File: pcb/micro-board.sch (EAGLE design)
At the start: 116 parts, among them IC1 STM32F401RET6U, IC2 LDS3985M33R, IC3 LDS3985M33R, IC4 HX711, IC5 TLV2462IP, J12 B2B-PH-K-S_LF__SN_, J14 3V3 LED, J15 VDDA LED, J16 HX711 LED, J18 DC Power, J3 Button / ADC Header, Q1 S8550, Q2 16MHz, U1 MCP73831.SOT23-5, U2 BR24S64FJ-WE2

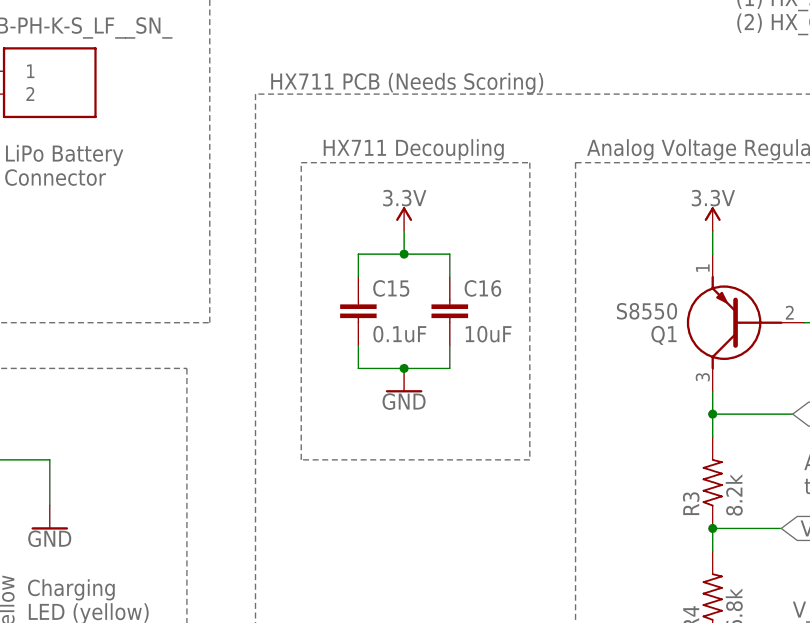
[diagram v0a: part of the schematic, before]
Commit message: Incremental commit of changes made
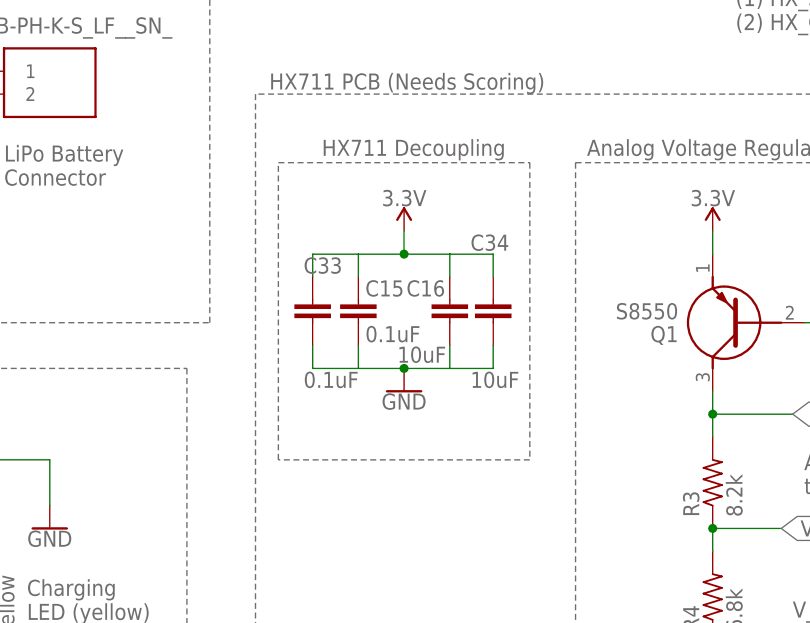
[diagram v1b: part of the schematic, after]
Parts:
- added C33: 0.1uF, LinnesLab-Passives:CAPACITOR0603
- added C34: 10uF, LinnesLab-Passives:CAPACITOR0603
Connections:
- net 3.3V: now also C33.1, C34.1
- net GND: now also C33.2, C34.2
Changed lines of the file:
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@@
 <setting verticaltext="up"/>
 </settings>
-<grid distance="0.1" unitdist="inch" unit="inch" style="lines" multiple="1" display="yes" altdistance="0.01" altunitdist="inch" altunit="inch"/>
+<grid distance="0.01" unitdist="inch" unit="inch" style="lines" multiple="1" display="yes" altdistance="0.01" altunitdist="inch" altunit="inch"/>
 <layers>
 <layer number="1" name="Top" color="4" fill="1" visible="no" active="no"/>
@@
 <part name="R39" library="LinnesLab-Passives" deviceset="RESISTOR" device="0603" package3d_urn="urn:adsk.eagle:package:15661944/2" value="10k"/>
 <part name="SUPPLY40" library="LinnesLab-Symbols" deviceset="3.3V" device=""/>
+<part name="C33" library="LinnesLab-Passives" deviceset="CAPACITOR" device="0603" package3d_urn="urn:adsk.eagle:package:15661989/2" value="0.1uF"/>
+<part name="C34" library="LinnesLab-Passives" deviceset="CAPACITOR" device="0603" package3d_urn="urn:adsk.eagle:package:15661989/2" value="10uF"/>
 </parts>
 <sheets>
@@
 <wire x1="363.22" y1="71.12" x2="363.22" y2="7.62" width="0.1524" layer="95" style="shortdash"/>
 <wire x1="363.22" y1="7.62" x2="414.02" y2="7.62" width="0.1524" layer="95" style="shortdash"/>
-<wire x1="332.74" y1="71.12" x2="358.14" y2="71.12" width="0.1524" layer="95" style="shortdash"/>
+<wire x1="330.2" y1="71.12" x2="358.14" y2="71.12" width="0.1524" layer="95" style="shortdash"/>
 <wire x1="358.14" y1="71.12" x2="358.14" y2="38.1" width="0.1524" layer="95" style="shortdash"/>
-<wire x1="358.14" y1="38.1" x2="332.74" y2="38.1" width="0.1524" layer="95" style="shortdash"/>
-<wire x1="332.74" y1="38.1" x2="332.74" y2="71.12" width="0.1524" layer="95" style="shortdash"/>
+<wire x1="358.14" y1="38.1" x2="330.2" y2="38.1" width="0.1524" layer="95" style="shortdash"/>
+<wire x1="330.2" y1="38.1" x2="330.2" y2="71.12" width="0.1524" layer="95" style="shortdash"/>
 <wire x1="327.66" y1="78.74" x2="327.66" y2="0" width="0.1524" layer="95" style="shortdash"/>
 <wire x1="327.66" y1="0" x2="553.72" y2="0" width="0.1524" layer="95" style="shortdash"/>
@@
 </instance>
 <instance part="C15" gate="G$1" x="339.09" y="53.34" smashed="yes">
-<attribute name="NAME" x="340.614" y="56.261" size="1.778" layer="95"/>
-<attribute name="VALUE" x="340.614" y="51.181" size="1.778" layer="96"/>
+<attribute name="NAME" x="339.852" y="56.261" size="1.778" layer="95"/>
+<attribute name="VALUE" x="339.852" y="51.181" size="1.778" layer="96"/>
 </instance>
 <instance part="C16" gate="G$1" x="349.25" y="53.34" smashed="yes">
-<attribute name="NAME" x="350.774" y="56.261" size="1.778" layer="95"/>
-<attribute name="VALUE" x="350.774" y="51.181" size="1.778" layer="96"/>
+<attribute name="NAME" x="344.424" y="56.261" size="1.778" layer="95"/>
+<attribute name="VALUE" x="343.408" y="48.895" size="1.778" layer="96"/>
 </instance>
 <instance part="GND18" gate="G$1" x="344.17" y="45.72" smashed="yes">
@@
 <attribute name="VALUE" x="246.38" y="155.194" size="1.778" layer="96" align="bottom-center"/>
 </instance>
+<instance part="C33" gate="G$1" x="334.01" y="53.34" smashed="yes">
+<attribute name="NAME" x="332.994" y="58.801" size="1.778" layer="95"/>
+<attribute name="VALUE" x="332.994" y="46.101" size="1.778" layer="96"/>
+</instance>
+<instance part="C34" gate="G$1" x="354.076" y="53.34" smashed="yes">
+<attribute name="NAME" x="351.536" y="61.341" size="1.778" layer="95"/>
+<attribute name="VALUE" x="351.536" y="46.101" size="1.778" layer="96"/>
+</instance>
 </instances>
 <busses>
@@
 <wire x1="349.25" y1="48.26" x2="344.17" y2="48.26" width="0.1524" layer="91"/>
 <junction x="344.17" y="48.26"/>
+<pinref part="C33" gate="G$1" pin="2"/>
+<wire x1="334.01" y1="50.8" x2="334.01" y2="48.26" width="0.1524" layer="91"/>
+<wire x1="334.01" y1="48.26" x2="339.09" y2="48.26" width="0.1524" layer="91"/>
+<pinref part="C34" gate="G$1" pin="2"/>
+<wire x1="354.076" y1="50.8" x2="354.076" y2="48.26" width="0.1524" layer="91"/>
+<wire x1="354.076" y1="48.26" x2="349.25" y2="48.26" width="0.1524" layer="91"/>
 </segment>
 <segment>
@@
 <wire x1="344.17" y1="60.96" x2="344.17" y2="63.5" width="0.1524" layer="91"/>
 <junction x="344.17" y="60.96"/>
-</segment>
-<segment>
+<pinref part="C33" gate="G$1" pin="1"/>
+<wire x1="334.01" y1="60.96" x2="334.01" y2="58.42" width="0.1524" layer="91"/>
+<wire x1="334.01" y1="60.96" x2="339.09" y2="60.96" width="0.1524" layer="91"/>
+<pinref part="C34" gate="G$1" pin="1"/>
+<wire x1="354.076" y1="58.42" x2="354.076" y2="60.96" width="0.1524" layer="91"/>
+<wire x1="354.076" y1="60.96" x2="349.25" y2="60.96" width="0.1524" layer="91"/>
+</segment>
+<segment>
